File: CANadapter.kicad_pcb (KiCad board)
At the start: 2 copper layers, 94 x 22.9 mm, 29 parts, among them P1 CONN_02X06, P2 CONN_01X06, P3 CONN_01X04, P4 CONN_01X06, U1 MCP2515, U2 TLP2361, U3 TLP2361, U4 MCP2551-I/SN, U5 LM7805CT, U6 NKE0305SC, Y1 16MHz

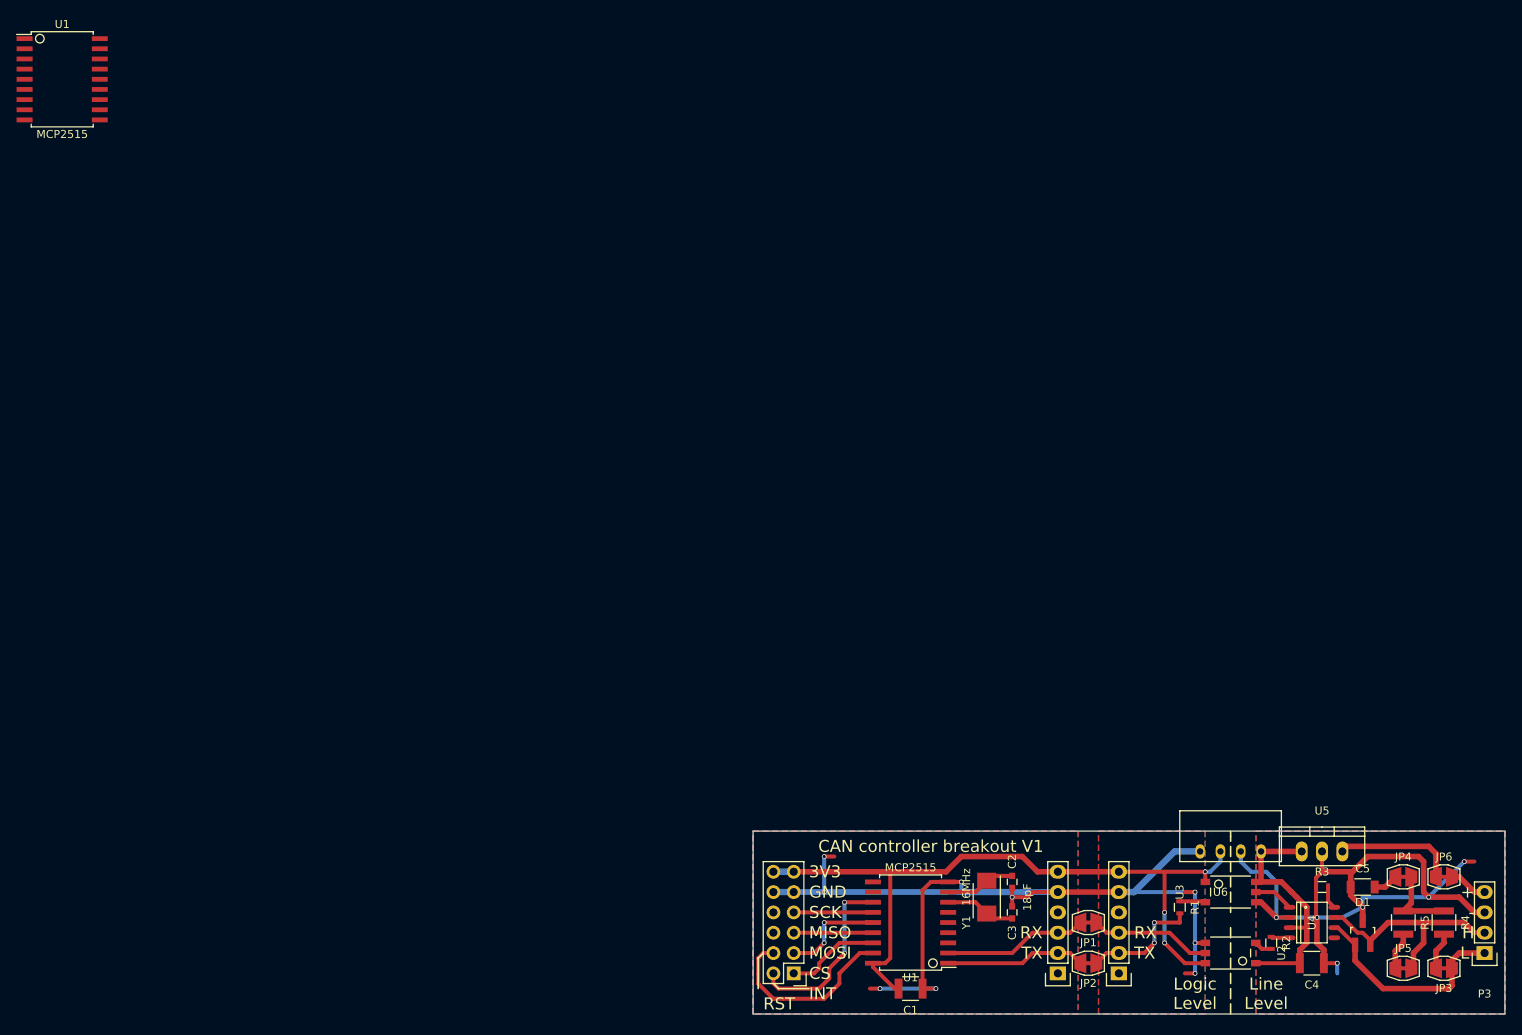
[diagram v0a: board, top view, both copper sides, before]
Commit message: improved silk
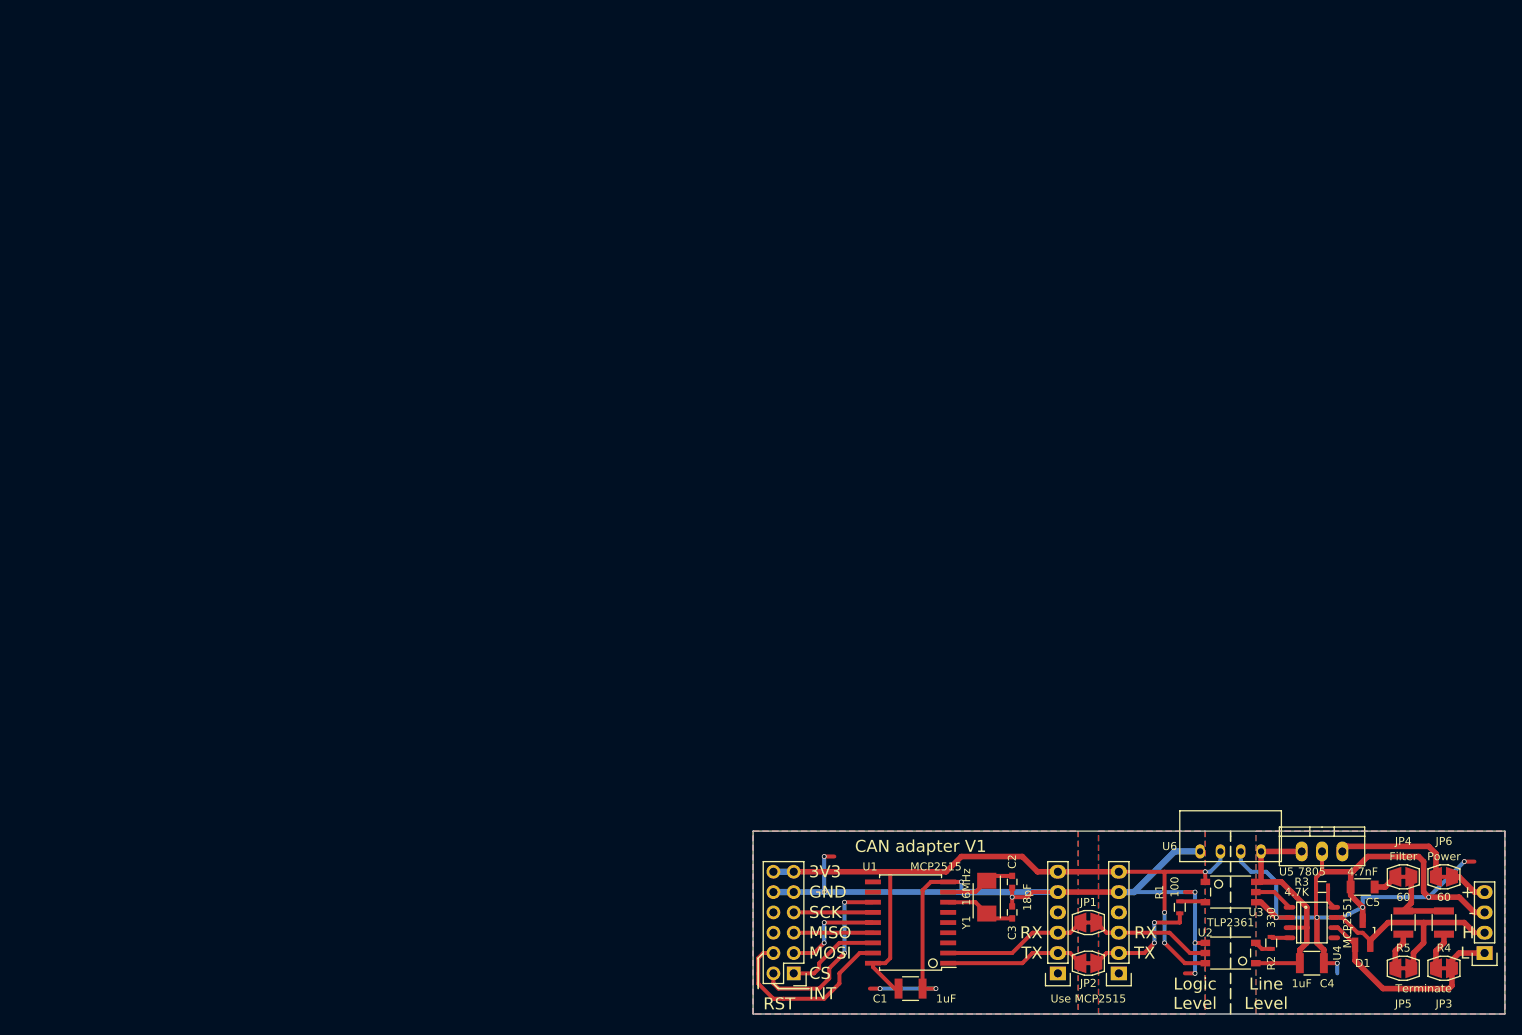
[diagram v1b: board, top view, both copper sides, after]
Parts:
- removed the U1 at (0.00, 0.00)
- JP6: value Line Power -> Power
- U4: value MCP2551-I/SN -> MCP2551
- U5: value LM7805CT -> 7805
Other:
- board text added: "CAN adapter V1"
